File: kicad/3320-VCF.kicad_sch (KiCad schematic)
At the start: 57 parts, among them J1 EuroPower_JST_3P, J2 EURO_PWR_16P, U1 TL072, U2 AS3320, U3 TL074

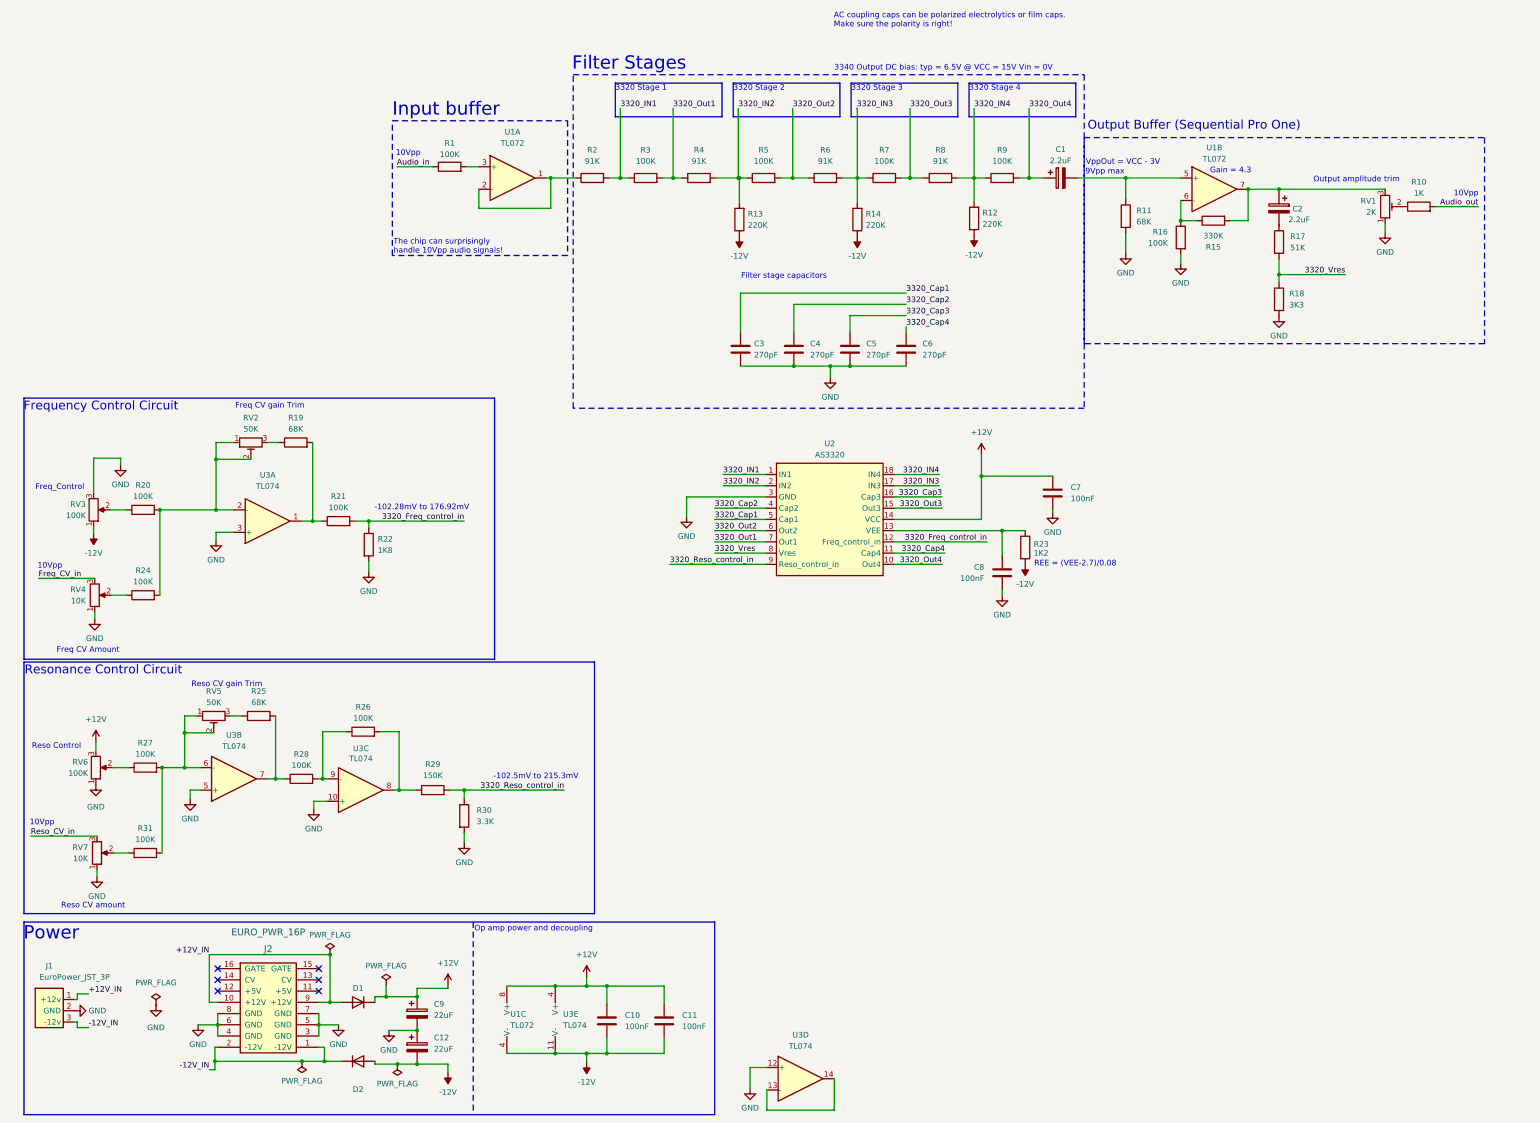
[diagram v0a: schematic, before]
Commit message: added schem rev 0.1.3
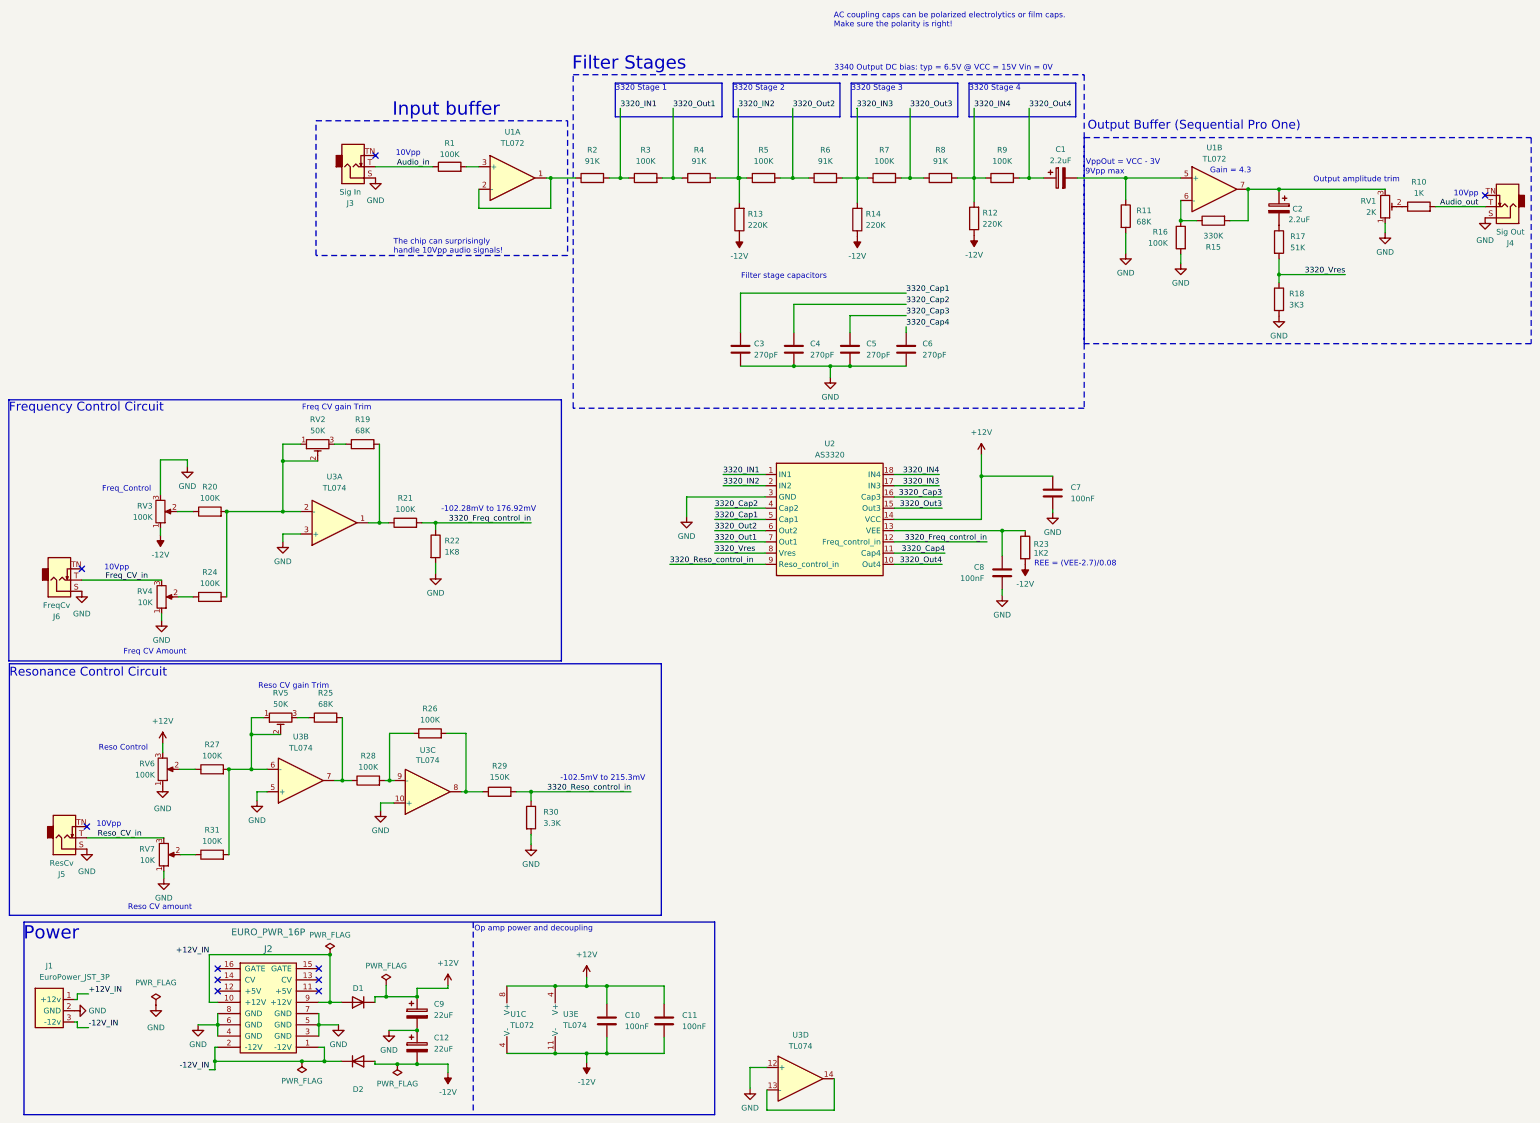
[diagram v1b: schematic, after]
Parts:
- added J3: Sig In, DIYSynthMNL:AudioJack_3.5mm_long_pads, symbol DIYSynthMNL:PJ3001F
- added J4: Sig Out, DIYSynthMNL:AudioJack_3.5mm_long_pads, symbol DIYSynthMNL:PJ3001F
- added J5: ResCv, DIYSynthMNL:AudioJack_3.5mm_long_pads, symbol DIYSynthMNL:PJ3001F
- added J6: FreqCv, DIYSynthMNL:AudioJack_3.5mm_long_pads, symbol DIYSynthMNL:PJ3001F
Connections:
- net Audio_in: now also J3.T
- net Audio_out: now also J4.T
- net Freq_CV_in: now also J6.T
- net GND: now also J3.S, J4.S, J5.S, J6.S
- net Reso_CV_in: now also J5.T
- no-connect marks 6 -> 10
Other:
- moved on the sheet: R19, R20, R21, R22, R24, R25, R26, R27, R28, R29, R30, R31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
